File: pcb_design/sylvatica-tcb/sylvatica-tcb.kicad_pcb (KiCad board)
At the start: 2 copper layers, 93 x 93 mm, 6 parts, among them J1 Conn_02x07_Odd_Even, J2 USB_C_Receptacle, J3 USB_C_Receptacle, J4 USB_C_Receptacle, J5 USB_C_Receptacle

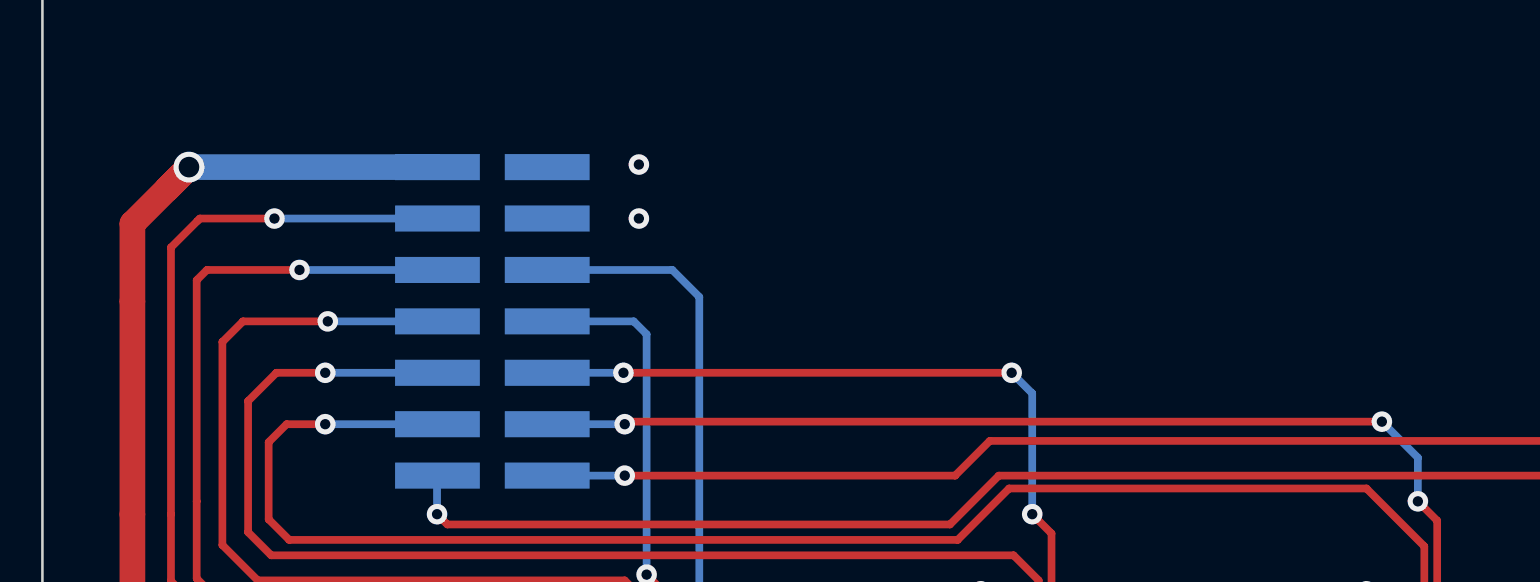
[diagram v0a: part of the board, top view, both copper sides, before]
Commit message: Various updates for Aisler order.
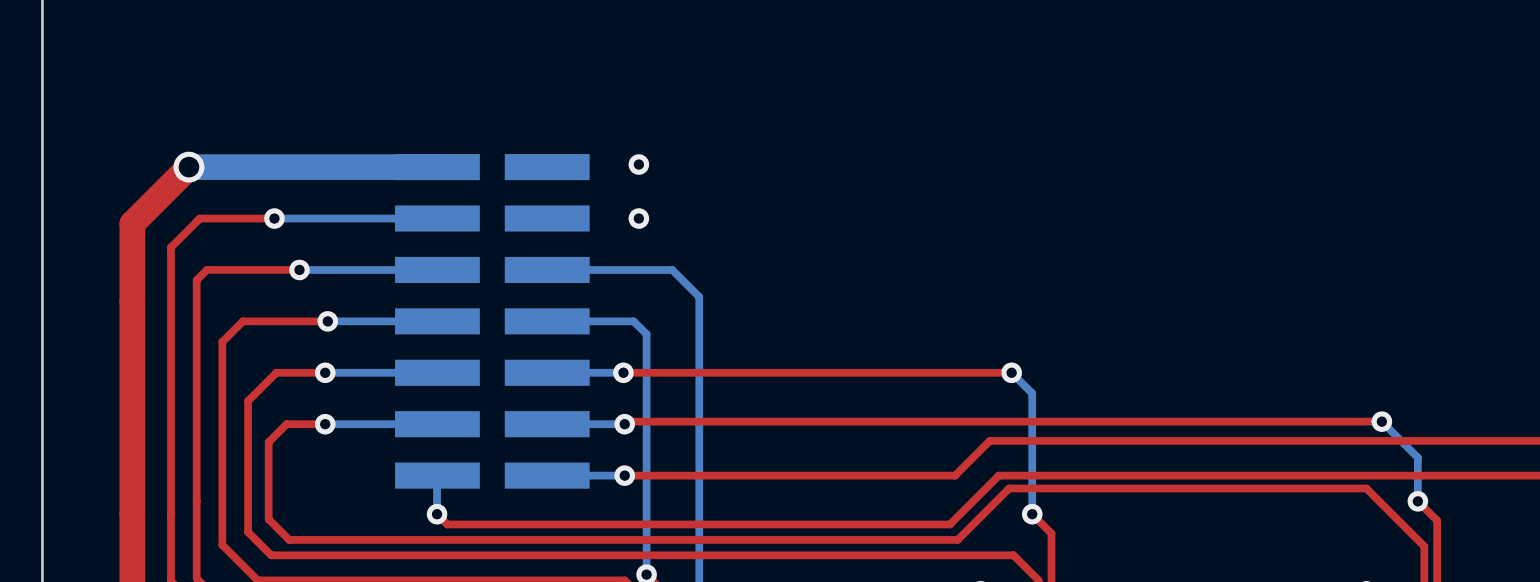
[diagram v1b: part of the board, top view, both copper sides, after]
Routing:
- net /S_PS2: track 153.7 -> 152.5 mm
